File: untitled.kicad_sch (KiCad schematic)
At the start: 128 parts, among them SW10 SW_Push, SW11 SW_Push, SW12 SW_Push, SW13 SW_Push, SW14 SW_Push, SW15 SW_Push, SW16 SW_Push, SW17 SW_Push, SW18 SW_Push, SW19 SW_Push, SW2 SW_Push, SW20 SW_Push, SW21 SW_Push, SW22 SW_Push, SW23 SW_Push, SW24 SW_Push, SW25 SW_Push, SW26 SW_Push, SW27 SW_Push, SW28 SW_Push, SW29 SW_Push, SW3 SW_Push, SW30 SW_Push, SW31 SW_Push, SW32 SW_Push, SW33 SW_Push, SW34 SW_Push, SW35 SW_Push, SW36 SW_Push, SW37 SW_Push, SW38 SW_Push, SW39 SW_Push, SW4 SW_Push, SW40 SW_Push, SW41 SW_Push, SW42 SW_Push, SW43 SW_Push, SW44 SW_Push, SW45 SW_Push, SW46 SW_Push, SW47 SW_Push, SW48 SW_Push, SW49 SW_Push, SW5 SW_Push, SW50 SW_Push, SW51 SW_Push, SW52 SW_Push, SW53 SW_Push, SW54 SW_Push, SW55 SW_Push, SW56 SW_Push, SW57 SW_Push, SW58 SW_Push, SW59 SW_Push, SW6 SW_Push, SW60 SW_Push, SW61 SW_Push, SW62 SW_Push, SW63 SW_Push, SW64 SW_Push, SW65 SW_Push, SW7 SW_Push, SW8 SW_Push, SW9 SW_Push

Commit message: Making.. 2
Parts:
- SW10, SW11, SW12, SW13, SW14, SW15, SW16, SW17, SW18, SW19, SW2, SW20, SW21, SW22, SW23, SW24, SW25, SW26, SW27, SW28, SW29, SW3, SW30, SW31, SW32, SW33, SW34, SW35, SW36, SW37, SW38, SW39, SW4, SW40, SW41, SW42, SW43, SW44, SW45, SW46, SW47, SW48, SW49, SW5, SW50, SW51, SW52, SW53, SW54, SW55, SW56, SW57, SW58, SW59, SW6, SW60, SW61, SW62, SW63, SW64, SW65, SW7, SW8, SW9: footprint keyswitches.pretty-2.1:Kailh_socket_MX -> PCM_Switch_Keyboard_Hotswap_Kailh:SW_Hotswap_Kailh_MX_1.00u

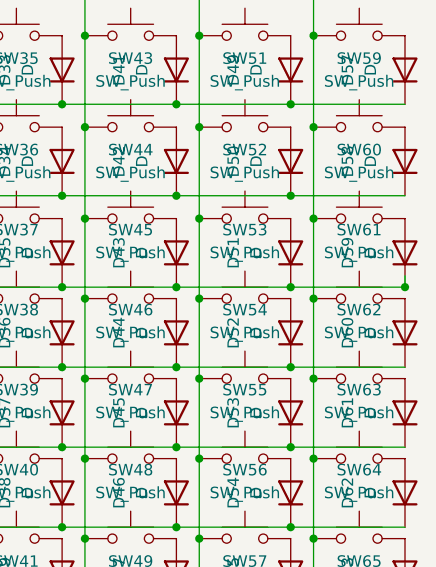
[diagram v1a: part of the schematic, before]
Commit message: making.... 3
making.... 3
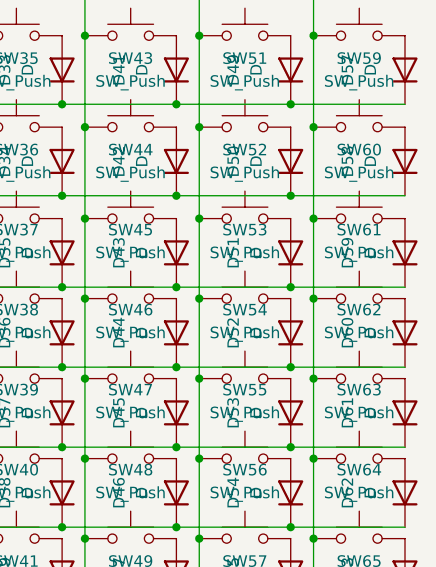
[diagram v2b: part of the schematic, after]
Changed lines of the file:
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@@
-	)
-	(junction
-		(at 250.19 64.77)
-		(diameter 0)
-		(color 0 0 0 0)
 	)
 	(junction
@@
 		)
 		(stroke
-			(width 0)
-			(type default)
-		)
-	)
-	(wire
-		(pts
-			(xy 250.19 63.5) (xy 250.19 64.77)
-		)
-		(stroke

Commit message: maybe final
maybe final
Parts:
- SW14, SW22, SW6: footprint PCM_Switch_Keyboard_Hotswap_Kailh:SW_Hotswap_Kailh_MX_1.00u -> PCM_Switch_Keyboard_Hotswap_Kailh:SW_Hotswap_Kailh_MX_1.25u
- SW3: footprint PCM_Switch_Keyboard_Hotswap_Kailh:SW_Hotswap_Kailh_MX_1.00u -> PCM_Switch_Keyboard_Hotswap_Kailh:SW_Hotswap_Kailh_MX_1.50u
- SW38: footprint PCM_Switch_Keyboard_Hotswap_Kailh:SW_Hotswap_Kailh_MX_1.00u -> PCM_Switch_Keyboard_Hotswap_Kailh:SW_Hotswap_Kailh_MX_6.25u
- SW4: footprint PCM_Switch_Keyboard_Hotswap_Kailh:SW_Hotswap_Kailh_MX_1.00u -> PCM_Switch_Keyboard_Hotswap_Kailh:SW_Hotswap_Kailh_MX_1.75u
- SW5, SW63: footprint PCM_Switch_Keyboard_Hotswap_Kailh:SW_Hotswap_Kailh_MX_1.00u -> PCM_Switch_Keyboard_Hotswap_Kailh:SW_Hotswap_Kailh_MX_2.00u
- SW64: footprint PCM_Switch_Keyboard_Hotswap_Kailh:SW_Hotswap_Kailh_MX_1.00u -> PCM_Switch_Keyboard_Hotswap_Kailh:SW_Hotswap_Kailh_MX_ISOEnter
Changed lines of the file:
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@@
 			)
 		)
-		(property "Footprint" "PCM_Switch_Keyboard_Hotswap_Kailh:SW_Hotswap_Kailh_MX_1.00u"
+		(property "Footprint" "PCM_Switch_Keyboard_Hotswap_Kailh:SW_Hotswap_Kailh_MX_2.00u"
 			(at 245.11 78.74 0)
 			(effects
@@
 			)
 		)
-		(property "Datasheet" "~"
+		(property "Datasheet" ""
 			(at 245.11 78.74 0)
 			(effects
@@
 			)
 		)
-		(property "Description" "Push button switch, generic, two pins"
+		(property "Description" ""
 			(at 245.11 83.82 0)
 			(effects
@@
 			)
 		)
-		(property "Footprint" "PCM_Switch_Keyboard_Hotswap_Kailh:SW_Hotswap_Kailh_MX_1.00u"
+		(property "Footprint" "PCM_Switch_Keyboard_Hotswap_Kailh:SW_Hotswap_Kailh_MX_6.25u"
 			(at 207.01 69.85 0)
 			(effects
@@
 			)
 		)
-		(property "Datasheet" "~"
+		(property "Datasheet" ""
 			(at 207.01 69.85 0)
 			(effects
@@
 			)
 		)
-		(property "Description" "Push button switch, generic, two pins"
+		(property "Description" ""
 			(at 207.01 74.93 0)
 			(effects
@@
 			)
 		)
-		(property "Footprint" "PCM_Switch_Keyboard_Hotswap_Kailh:SW_Hotswap_Kailh_MX_1.00u"
+		(property "Footprint" "PCM_Switch_Keyboard_Hotswap_Kailh:SW_Hotswap_Kailh_MX_1.75u"
 			(at 157.48 52.07 0)
 			(effects
@@
 			)
 		)
-		(property "Datasheet" "~"
+		(property "Datasheet" ""
 			(at 157.48 52.07 0)
 			(effects
@@
 			)
 		)
-		(property "Description" "Push button switch, generic, two pins"
+		(property "Description" ""
 			(at 157.48 57.15 0)
 			(effects
@@
 			)
 		)
-		(property "Footprint" "PCM_Switch_Keyboard_Hotswap_Kailh:SW_Hotswap_Kailh_MX_1.00u"
+		(property "Footprint" "PCM_Switch_Keyboard_Hotswap_Kailh:SW_Hotswap_Kailh_MX_2.00u"
 			(at 157.48 60.96 0)
 			(effects
@@
 			)
 		)
-		(property "Datasheet" "~"
+		(property "Datasheet" ""
 			(at 157.48 60.96 0)
 			(effects
@@
 			)
 		)
-		(property "Description" "Push button switch, generic, two pins"
+		(property "Description" ""
 			(at 157.48 66.04 0)
 			(effects
@@
 			)
 		)
-		(property "Footprint" "PCM_Switch_Keyboard_Hotswap_Kailh:SW_Hotswap_Kailh_MX_1.00u"
+		(property "Footprint" "PCM_Switch_Keyboard_Hotswap_Kailh:SW_Hotswap_Kailh_MX_1.25u"
 			(at 157.48 69.85 0)
 			(effects
@@
 			)
 		)
-		(property "Datasheet" "~"
+		(property "Datasheet" ""
 			(at 157.48 69.85 0)
 			(effects
@@
 			)
 		)
-		(property "Description" "Push button switch, generic, two pins"
+		(property "Description" ""
 			(at 157.48 74.93 0)
 			(effects
@@
 			)
 		)
-		(property "Footprint" "PCM_Switch_Keyboard_Hotswap_Kailh:SW_Hotswap_Kailh_MX_1.00u"
+		(property "Footprint" "PCM_Switch_Keyboard_Hotswap_Kailh:SW_Hotswap_Kailh_MX_ISOEnter"
 			(at 245.11 87.63 0)
 			(effects
@@
 			)
 		)
-		(property "Datasheet" "~"
+		(property "Datasheet" ""
 			(at 245.11 87.63 0)
 			(effects
@@
 			)
 		)
-		(property "Description" "Push button switch, generic, two pins"
+		(property "Description" ""
 			(at 245.11 92.71 0)
 			(effects
@@
 			)
 		)
-		(property "Footprint" "PCM_Switch_Keyboard_Hotswap_Kailh:SW_Hotswap_Kailh_MX_1.00u"
+		(property "Footprint" "PCM_Switch_Keyboard_Hotswap_Kailh:SW_Hotswap_Kailh_MX_1.25u"
 			(at 168.91 69.85 0)
 			(effects
@@
 			)
 		)
-		(property "Datasheet" "~"
+		(property "Datasheet" ""
 			(at 168.91 69.85 0)
 			(effects
@@
 			)
 		)
-		(property "Description" "Push button switch, generic, two pins"
+		(property "Description" ""
 			(at 168.91 74.93 0)
 			(effects
@@
 			)
 		)
-		(property "Footprint" "PCM_Switch_Keyboard_Hotswap_Kailh:SW_Hotswap_Kailh_MX_1.00u"
+		(property "Footprint" "PCM_Switch_Keyboard_Hotswap_Kailh:SW_Hotswap_Kailh_MX_1.25u"
 			(at 181.61 69.85 0)
 			(effects
@@
 			)
 		)
-		(property "Datasheet" "~"
+		(property "Datasheet" ""
 			(at 181.61 69.85 0)
 			(effects
@@
 			)
 		)
-		(property "Description" "Push button switch, generic, two pins"
+		(property "Description" ""
 			(at 181.61 74.93 0)
 			(effects
@@
 			)
 		)
-		(property "Footprint" "PCM_Switch_Keyboard_Hotswap_Kailh:SW_Hotswap_Kailh_MX_1.00u"
+		(property "Footprint" "PCM_Switch_Keyboard_Hotswap_Kailh:SW_Hotswap_Kailh_MX_1.50u"
 			(at 157.48 41.91 0)
 			(effects
@@
 			)
 		)
-		(property "Datasheet" "~"
+		(property "Datasheet" ""
 			(at 157.48 41.91 0)
 			(effects
@@
 			)
 		)
-		(property "Description" "Push button switch, generic, two pins"
+		(property "Description" ""
 			(at 157.48 46.99 0)
 			(effects
